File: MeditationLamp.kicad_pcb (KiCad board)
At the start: 2 copper layers, 18.9 x 81.8 mm, 8 parts, among them J1 Conn_01x03_Male, SW1 SW_SPST, U1 ATmega328-P

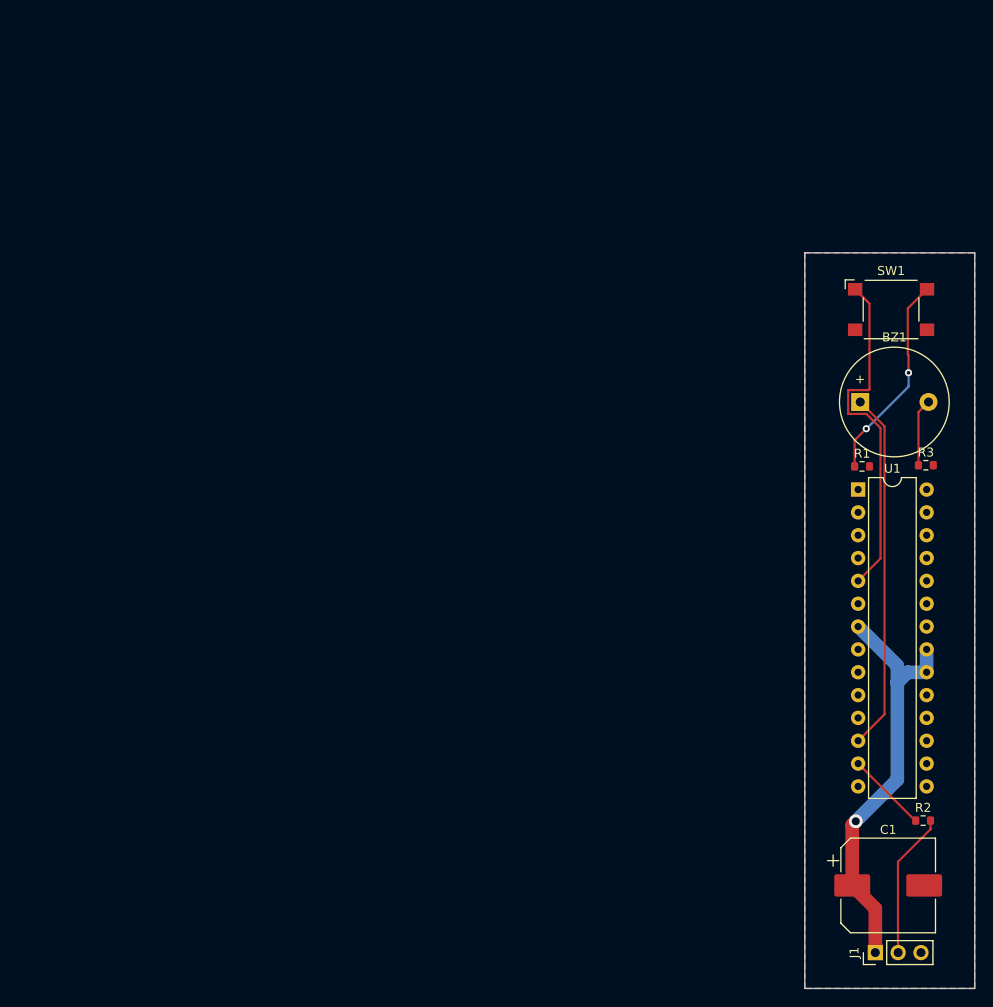
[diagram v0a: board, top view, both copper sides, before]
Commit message: add gerbers
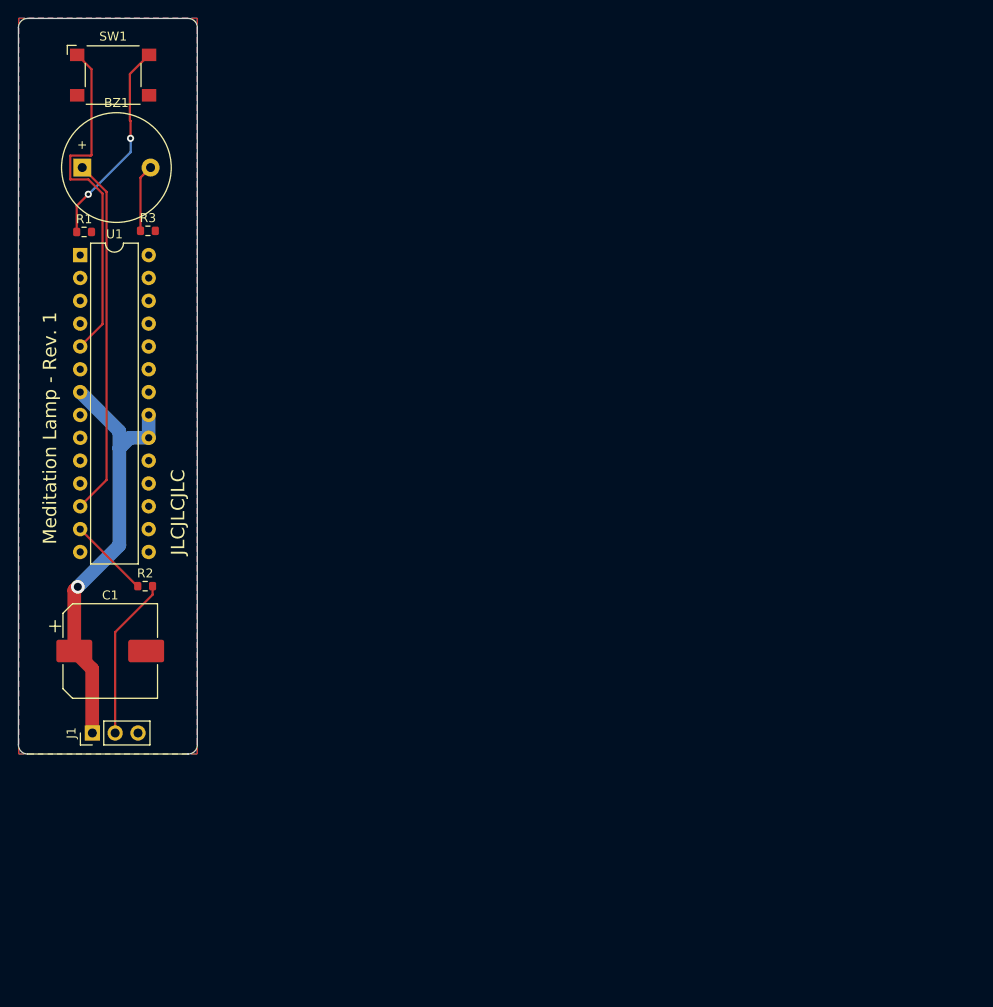
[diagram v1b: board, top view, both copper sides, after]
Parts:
- moved J1 90.4 mm to (28.2, 99.5)
- moved BZ1 90.4 mm to (27.1, 36.6)
- moved C1 90.4 mm to (30.2, 90.4)
- moved R1 90.4 mm to (27.3, 43.8)
- moved R2 90.4 mm to (34.1, 83.2)
- moved R3 90.4 mm to (34.4, 43.6)
- moved SW1 90.4 mm to (30.5, 26.3)
- moved U1 90.4 mm to (26.9, 46.3)
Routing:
- net Net-(J1-Pad2): track 16.2 -> 18.1 mm
- net +5V: track 47.5 -> 48.9 mm
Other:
- board size 18.9 x 81.8 mm -> 19.9 x 81.8 mm
- board text added: "JLCJLCJLC"
- board text added: "Meditation Lamp - Rev. 1"
